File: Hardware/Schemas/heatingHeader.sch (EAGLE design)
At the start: 26 parts, among them IC1 DS1820

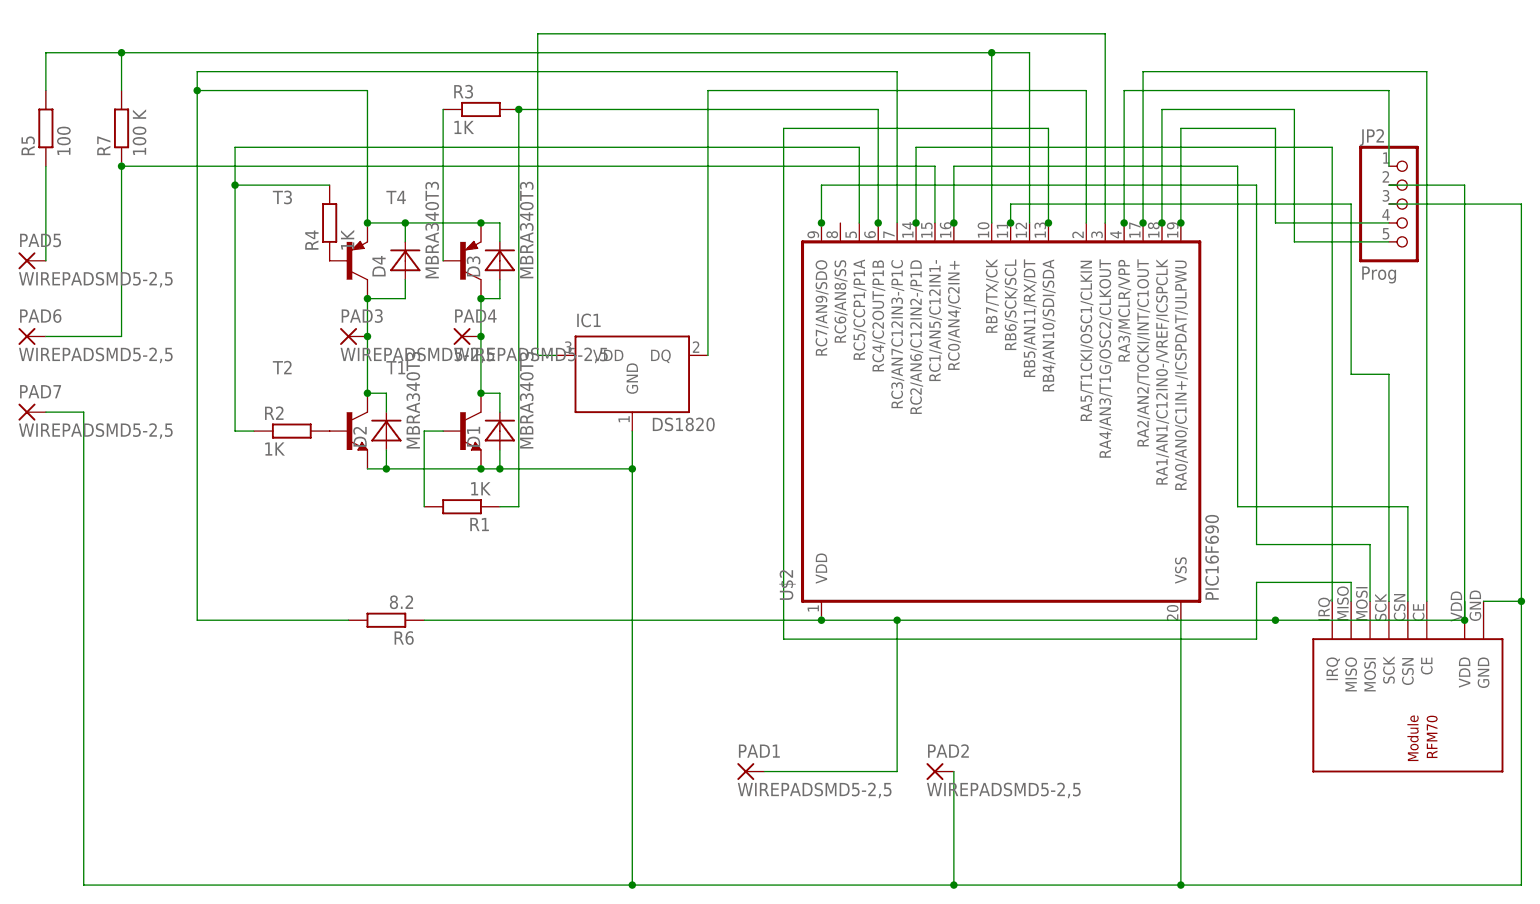
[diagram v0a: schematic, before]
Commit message: a
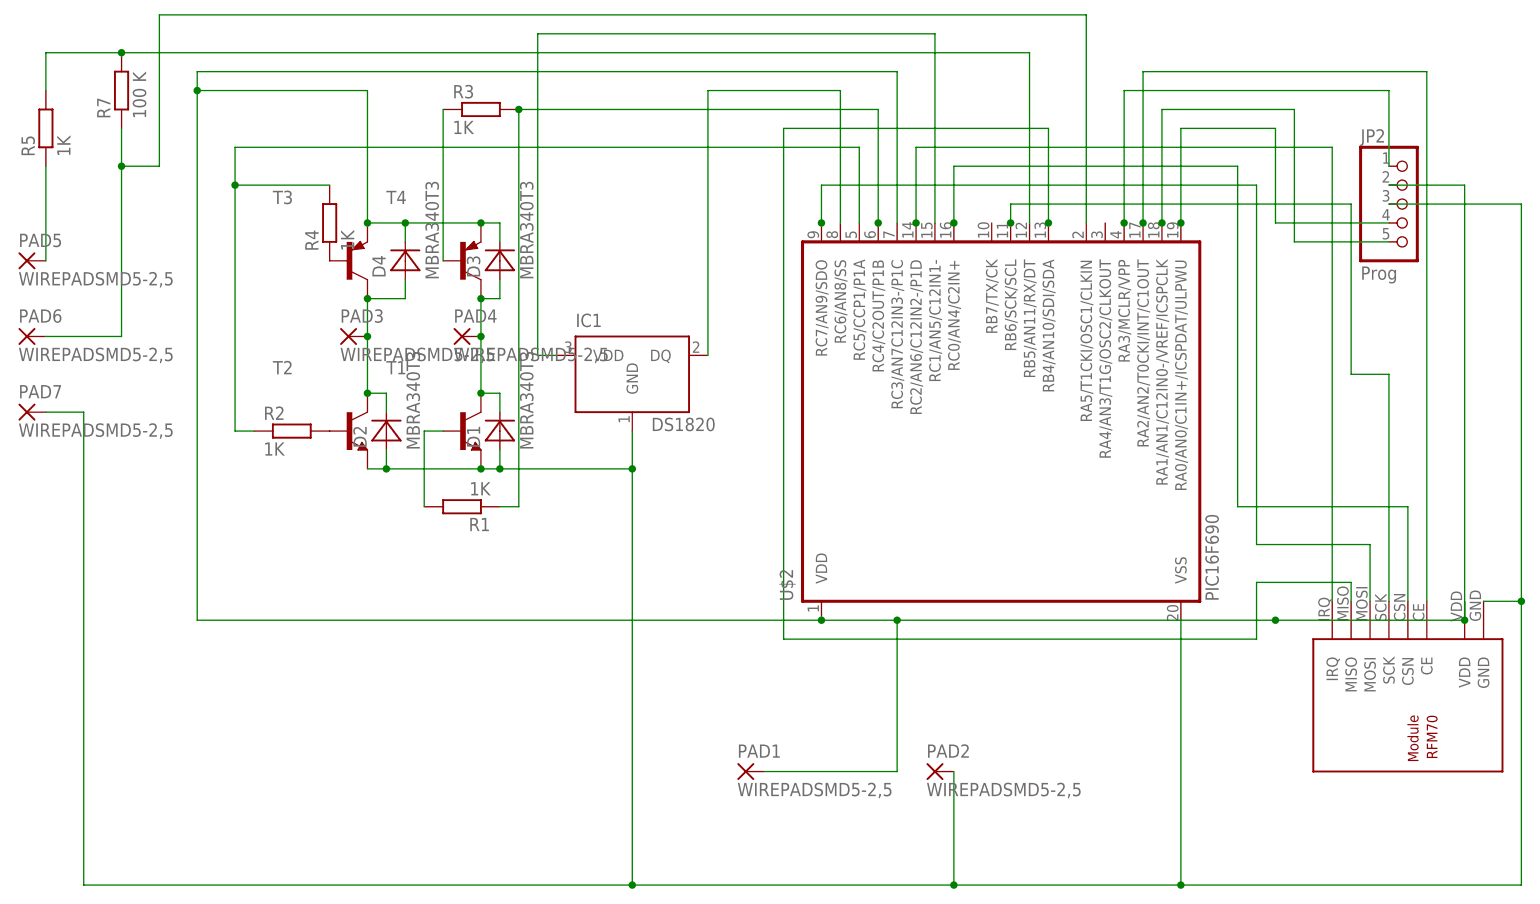
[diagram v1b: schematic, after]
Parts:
- removed R6: 8.2, resistor:R-EU_R6332
- R5: value 100 -> 1K
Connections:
- removed net N$11: PAD6.P, R7.1, U$2.RC1/AN5/C12IN1-
- removed net N$17: JP2.2, PAD1.P, R6.1, U$1.VDD, U$2.VDD
- new net N$9: PAD6.P, R7.1, U$2.RA5/T1CKI/OSC1/CLKIN
- net N$1: now also U$2.RC6/AN8/SS; no longer U$2.RA5/T1CKI/OSC1/CLKIN
- net N$2: now also JP2.2, PAD1.P, U$1.VDD, U$2.VDD; no longer R6.2
- net N$28: no longer U$2.RB7/TX/CK
- net N$3: now also U$2.RC1/AN5/C12IN1-; no longer U$2.RA4/AN3/T1G/OSC2/CLKOUT
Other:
- moved on the sheet: R7
